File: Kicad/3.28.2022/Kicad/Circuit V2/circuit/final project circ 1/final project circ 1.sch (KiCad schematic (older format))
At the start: 61 parts, among them J1 Conn_01x04_Female, J10 Conn_01x02_Female, J11 Conn_01x03_Female, J2 Conn_01x01_Female, J3 Conn_01x04_Female, J4 Conn_01x04_Female, J5 Conn_01x03_Female, J6 Conn_01x03_Female, J7 Conn_01x03_Female, J8 Conn_01x02_Female, J9 Conn_01x02_Female, Q1 FDD770N15A, Q2 FDD770N15A, Q3 FDD770N15A, Q6 2SC1945, U1 LTC3895IFE, U2 ESP32-DEVKITC-32D, U5 AZ1117-3.3, U7 SRD-S-112DM, U8 L2293QTR

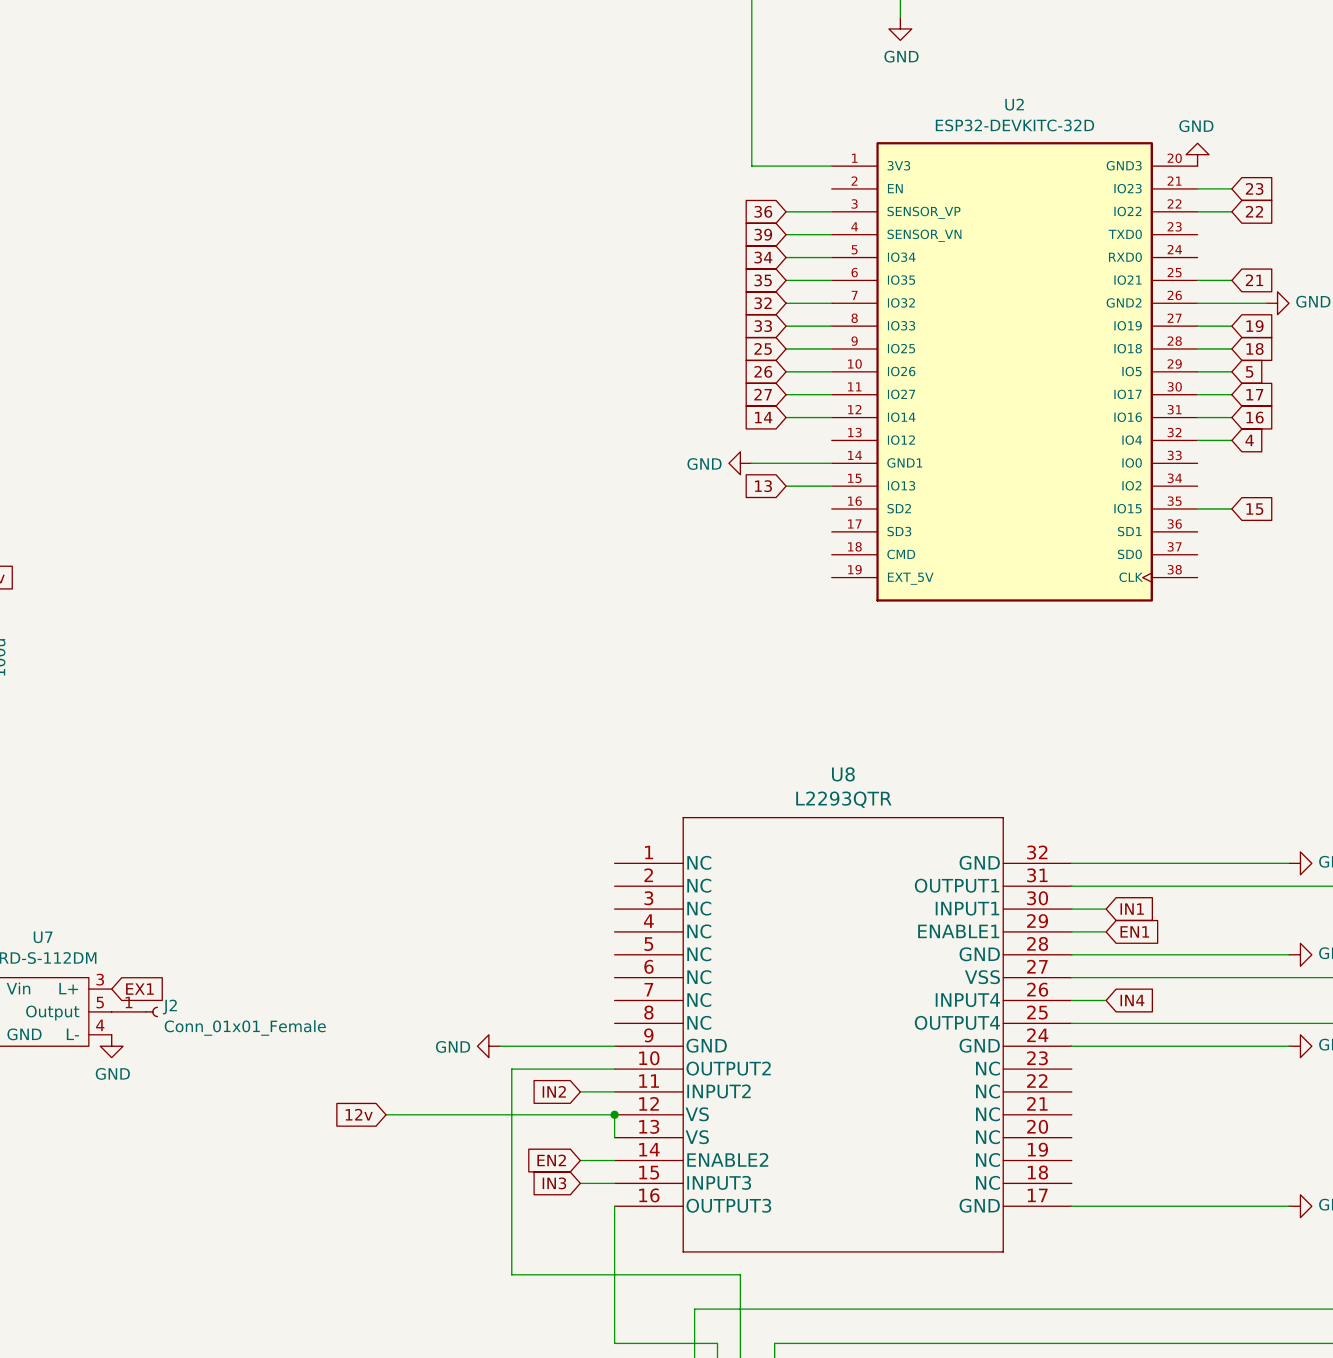
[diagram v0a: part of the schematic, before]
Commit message: Finished logic circit
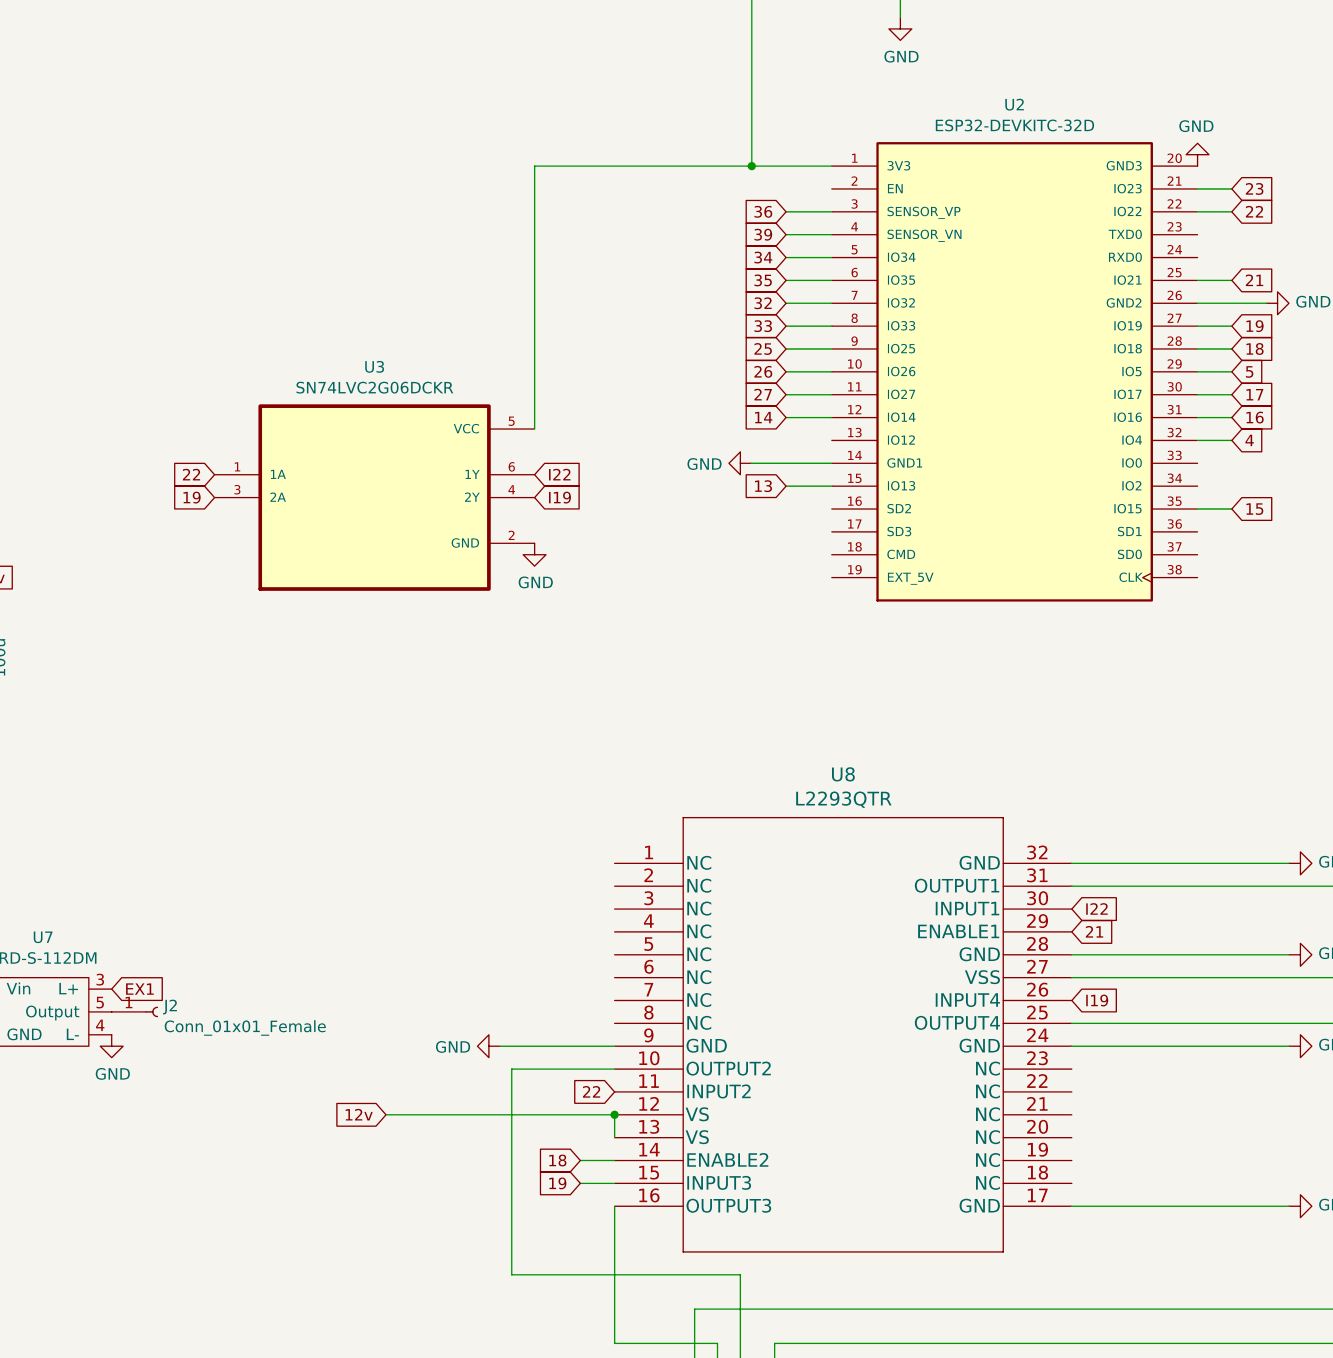
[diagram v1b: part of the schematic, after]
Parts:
- added U3: SN74LVC2G06DCKR, SOT65P210X110-6N, symbol Custom:SN74LVC2G06DCKR
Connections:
- net EN1 is gone; now on net 21: U8.29 (ENABLE1)
- net EN2 is gone; now on net 18: U8.14 (ENABLE2)
- net IN2 is gone; now on net 22: U8.11 (INPUT2)
- net IN3 is gone; now on net 19: U8.15 (INPUT3)
- net 19: now also U3.3 (2A)
- net 22: now also U3.1 (1A)
- net GND: now also U3.2 (GND)
- net Volt33: now also U3.5 (VCC)
- net IN1 renamed I22
- net I22: now also U3.6 (1Y)
- net IN4 renamed I19
- net I19: now also U3.4 (2Y)
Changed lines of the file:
@@
 Wire Wire Line
 	24300 18950 25250 18950
-Text GLabel 24450 17750 2    50   Input ~ 0
-EN1
-Text GLabel 22150 18750 0    50   Input ~ 0
-EN2
-Wire Wire Line
-	24300 17750 24450 17750
 Wire Wire Line
 	22150 18750 22300 18750
-Text GLabel 24450 17650 2    50   Input ~ 0
-IN1
-Text GLabel 22150 18450 0    50   Input ~ 0
-IN2
-Text GLabel 22150 18850 0    50   Input ~ 0
-IN3
-Text GLabel 24450 18050 2    50   Input ~ 0
-IN4
-Wire Wire Line
-	24300 17650 24450 17650
-Wire Wire Line
-	24450 18050 24300 18050
-Wire Wire Line
-	22150 18450 22300 18450
 Wire Wire Line
 	22150 18850 22300 18850
@@
 Wire Wire Line
 	23050 15500 23250 15500
+$Comp
+L Custom:SN74LVC2G06DCKR U3
+U 1 1 624C81FC
+P 21250 15850
+F 0 "U3" H 21250 16420 50  0000 C CNN
+F 1 "SN74LVC2G06DCKR" H 21250 16329 50  0000 C CNN
+F 2 "SOT65P210X110-6N" H 21250 15850 50  0001 L BNN
+F 3 "" H 21250 15850 50  0001 L BNN
+	1    21250 15850
+	1    0    0    -1
+$EndComp
+Wire Wire Line
+	22900 14400 21950 14400
+Wire Wire Line
+	21950 14400 21950 15550
+Connection ~ 22900 14400
+$Comp
+L power:GND #PWR033
+U 1 1 624DE9E3
+P 21950 16050
+F 0 "#PWR033" H 21950 15800 50  0001 C CNN
+F 1 "GND" H 21955 15877 50  0000 C CNN
+F 2 "" H 21950 16050 50  0001 C CNN
+F 3 "" H 21950 16050 50  0001 C CNN
+	1    21950 16050
+	1    0    0    -1
+$EndComp
+Text GLabel 24300 17750 2    50   Input ~ 0
+21
+Text GLabel 22150 18750 0    50   Input ~ 0
+18
+Text GLabel 20550 15750 0    50   Input ~ 0
+22
+Text GLabel 20550 15850 0    50   Input ~ 0
+19
+Text GLabel 22150 18850 0    50   Input ~ 0
+19
+Text GLabel 21950 15750 2    50   Input ~ 0
+I22
+Text GLabel 21950 15850 2    50   Input ~ 0
+I19
+Text GLabel 24300 18050 2    50   Input ~ 0
+I19
+Text GLabel 22300 18450 0    50   Input ~ 0
+22
+Text GLabel 24300 17650 2    50   Input ~ 0
+I22
 $EndSCHEMATC

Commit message: circ update
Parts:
- removed A1, A2, A3: Pololu_Breakout_DRV8825, Module:Pololu_Breakout-16_15.2x20.3mm, symbol Driver_Motor:Pololu_Breakout_DRV8825
- removed J3: Conn_01x04_Female, Connector_PinSocket_2.54mm:PinSocket_1x04_P2.54mm_Vertical, symbol Connector:Conn_01x04_Female
- added D? (x2): LED, symbol Device:LED
- added J12, J13: Conn_01x04_Female, symbol Connector:Conn_01x04_Female
- added J14: Barrel_Jack, symbol Connector:Barrel_Jack
- added J3: Conn_01x02_Female, symbol Connector:Conn_01x02_Female
- added Q?: BC337, Package_TO_SOT_THT:TO-92_Inline, symbol Transistor_BJT:BC337
- added R?: 20 ohm, symbol Device:R
- added R?: 150 ohm, symbol Device:R
- added R? (x6): Ohm, symbol Device:R
- added U4, U6, U9: A4988_STEPPER_MOTOR_DRIVER_CARRIER, symbol Custom:A4988_STEPPER_MOTOR_DRIVER_CARRIER
- C1, C5: footprint Capacitor_SMD:C_1210_3225Metric -> (none)
- C10, C13, C8, C9: footprint Capacitor_THT:CP_Radial_D6.3mm_P2.50mm -> (none)
- C11, C12: footprint Capacitor_THT:CP_Radial_D16.0mm_P7.50mm -> (none)
- C2: footprint Capacitor_SMD:C_0603_1608Metric -> (none)
- C21: footprint Capacitor_Tantalum_SMD:CP_EIA-3528-21_Kemet-B -> (none)
- C22, C3, C4, C6: footprint Capacitor_SMD:C_1206_3216Metric -> (none)
- C23: footprint Capacitor_Tantalum_SMD:CP_EIA-7343-40_Kemet-Y -> (none)
- C7: footprint Capacitor_SMD:C_0805_2012Metric -> (none)
- D1, D2, D3, D4, D5: footprint Diode_THT:D_DO-41_SOD81_P10.16mm_Horizontal -> (none)
- D9: footprint bigboard:SMAJ140CA -> (none)
- J1, J4: footprint Connector_PinSocket_2.54mm:PinSocket_1x04_P2.54mm_Vertical -> (none)
- J10, J8, J9: footprint bigboard:button -> (none)
- J11, J5, J6, J7: footprint bigboard:encoder_out -> (none)
- L1: footprint bigboard:MPXV1D1740L330 -> (none)
- PWM1, PWM2: footprint Connector_PinSocket_2.54mm:PinSocket_1x02_P2.54mm_Vertical -> (none)
- Q1, Q2, Q3, U5: footprint Package_TO_SOT_SMD:TO-252-3_TabPin2 -> (none)
- Q6: footprint Package_TO_SOT_THT:TO-220-3_Vertical -> (none)
- R1, R17, R18, R19, R20, R21, R22, R23: footprint Resistor_SMD:R_1210_3225Metric -> (none)
- R2, R3, R5: footprint Resistor_SMD:R_0805_2012Metric -> (none)
- R4: footprint Resistor_SMD:R_0603_1608Metric -> (none)
- R8: footprint Resistor_THT:R_Axial_DIN0309_L9.0mm_D3.2mm_P12.70mm_Horizontal -> (none)
- U1: footprint bigboard:LTC3895IFE -> (none)
- U2: footprint MODULE_ESP32-DEVKITC-32D -> (none)
- U3: footprint SOT65P210X110-6N -> (none)
- U7: footprint bigboard:SRD-S-112DM(F-11) Relay -> (none)
- U8: footprint bigboard:L2293QTR -> (none)
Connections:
- net 12v: now also R?.1, R?.1, U4.16 (VMOT), U6.16 (VMOT), U9.16 (VMOT)
- net 13: now also J11.2 (Pin_2); no longer J11.3 (Pin_3)
- net 19: now also R?.1
- net 22: now also R?.1
- net 23: now also U9.7 (STEP)
- net 25: now also U9.8 (DIR)
- net 26: now also U6.7 (STEP)
- net 27: now also U6.8 (DIR)
- net 32: now also U4.7 (STEP)
- net 33: now also U4.8 (DIR)
- net 4: now also J7.2 (Pin_2); no longer J7.3 (Pin_3)
- net GND: now also D?.1 (K), D?.1 (K), Q?.3 (E), R?.1, U4.15 (GND), U4.9 (GND), U6.15 (GND), U6.9 (GND), U9.15 (GND), U9.9 (GND)
- net I19: now also R?.1
- net I22: now also R?.1
- net Volt33: now also J11.3 (Pin_3), J7.3 (Pin_3), R?.2, U4.10 (VDD), U6.10 (VDD), U9.10 (VDD); no longer J11.2 (Pin_2), J7.2 (Pin_2)
- net at J4.2 (Pin_2): now also U4.11 (1B)
- net at J4.1 (Pin_1): now also U4.12 (1A)
- net at J4.3 (Pin_3): now also U4.13 (2A)
- net at J4.4 (Pin_4): now also U4.14 (2B)
- net at J1.2 (Pin_2): now also R?.2
- net at J1.1 (Pin_1): now also R?.2
- net at J1.3 (Pin_3): now also R?.2
- net at J1.4 (Pin_4): now also R?.2
- net EX1: no longer names the net of U7.3 (L+)
- net EX1: now also Q?.1 (C)
- new net: J3.1 (Pin_1), R?.2
- new net: J3.2 (Pin_2), R?.2
- new net: U4.5 (~RESET), U4.6 (~SLEEP)
- new net: J12.2 (Pin_2), U6.11 (1B)
- new net: J12.1 (Pin_1), U6.12 (1A)
- new net: J12.3 (Pin_3), U6.13 (2A)
- new net: J12.4 (Pin_4), U6.14 (2B)
- new net: U6.5 (~RESET), U6.6 (~SLEEP)
- new net: J13.2 (Pin_2), U9.11 (1B)
- new net: J13.1 (Pin_1), U9.12 (1A)
- new net: J13.3 (Pin_3), U9.13 (2A)
- new net: J13.4 (Pin_4), U9.14 (2B)
- new net: U9.5 (~RESET), U9.6 (~SLEEP)
- new net: D?.2 (A), R?.2
- new net: D?.2 (A), R?.1
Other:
- note added: "Analog 1\n"
- note added: "Analog 2"
- note added: "Backup pins for pwm\n"
- note added: "Button 1\n"
- note added: "Button 2\n"
- note added: "Button 3\n"
- note added: "Encoder 2\n"
- note added: "Encoder1\n"
- note added: "Motor driver/pwm"
- moved on the sheet: C1, C10, C11, C12, C13, C2, C3, C4, C5, C6, C7, C8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
